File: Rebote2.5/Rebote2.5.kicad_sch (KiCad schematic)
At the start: 51 parts, among them U1 TL072, U2 L78L05_TO92, U3 PT2399

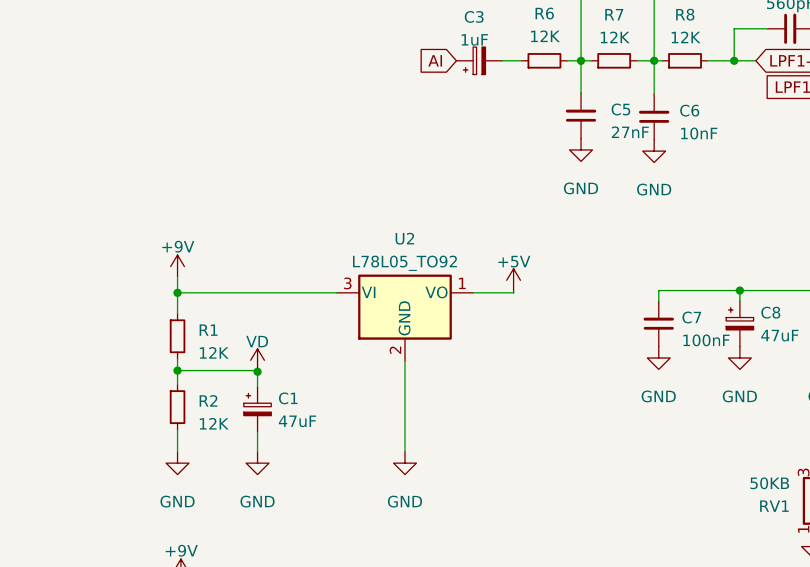
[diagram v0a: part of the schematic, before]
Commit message: WIP
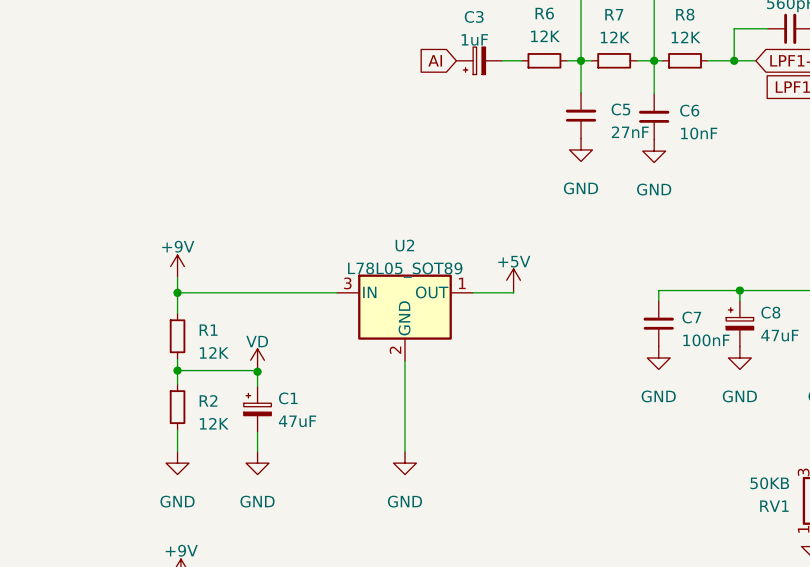
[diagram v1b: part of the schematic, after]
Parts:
- removed U2: L78L05_TO92, Package_TO_SOT_THT:TO-92_Inline, symbol Regulator_Linear:L78L05_TO92
- added U2: L78L05_SOT89, Package_TO_SOT_SMD:SOT-89-3, symbol Regulator_Linear:L78L05_SOT89
- C12, C13, C14, C15, C17, C18, C19, C2, C20, C25, C26, C4, C5, C6, C7, C9: footprint Capacitor_THT:C_Rect_L7.0mm_W3.5mm_P2.50mm_P5.00mm -> Capacitor_SMD:C_0805_2012Metric_Pad1.18x1.45mm_HandSolder
- R1, R10, R11, R12, R13, R14, R15, R16, R17, R18, R19, R2, R20, R21, R3, R4, R5, R6, R7, R8, R9: footprint Resistor_THT:R_Axial_DIN0207_L6.3mm_D2.5mm_P7.62mm_Horizontal -> Resistor_SMD:R_0805_2012Metric_Pad1.20x1.40mm_HandSolder
- U1: footprint Package_DIP:DIP-8_W7.62mm -> Package_SO:SOIC-8_3.9x4.9mm_P1.27mm
- U3: footprint Package_DIP:DIP-16_W7.62mm -> Package_SO:SOIC-16_3.9x9.9mm_P1.27mm
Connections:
- net +5V: now also U2.1 (OUT)
- net +9V: now also U2.3 (IN)
- net GND: now also U2.2 (GND)
